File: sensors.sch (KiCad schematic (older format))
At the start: 23 parts, among them M1 ANEOMETER, U2 ADS1120-PW, U5 MPL115A1

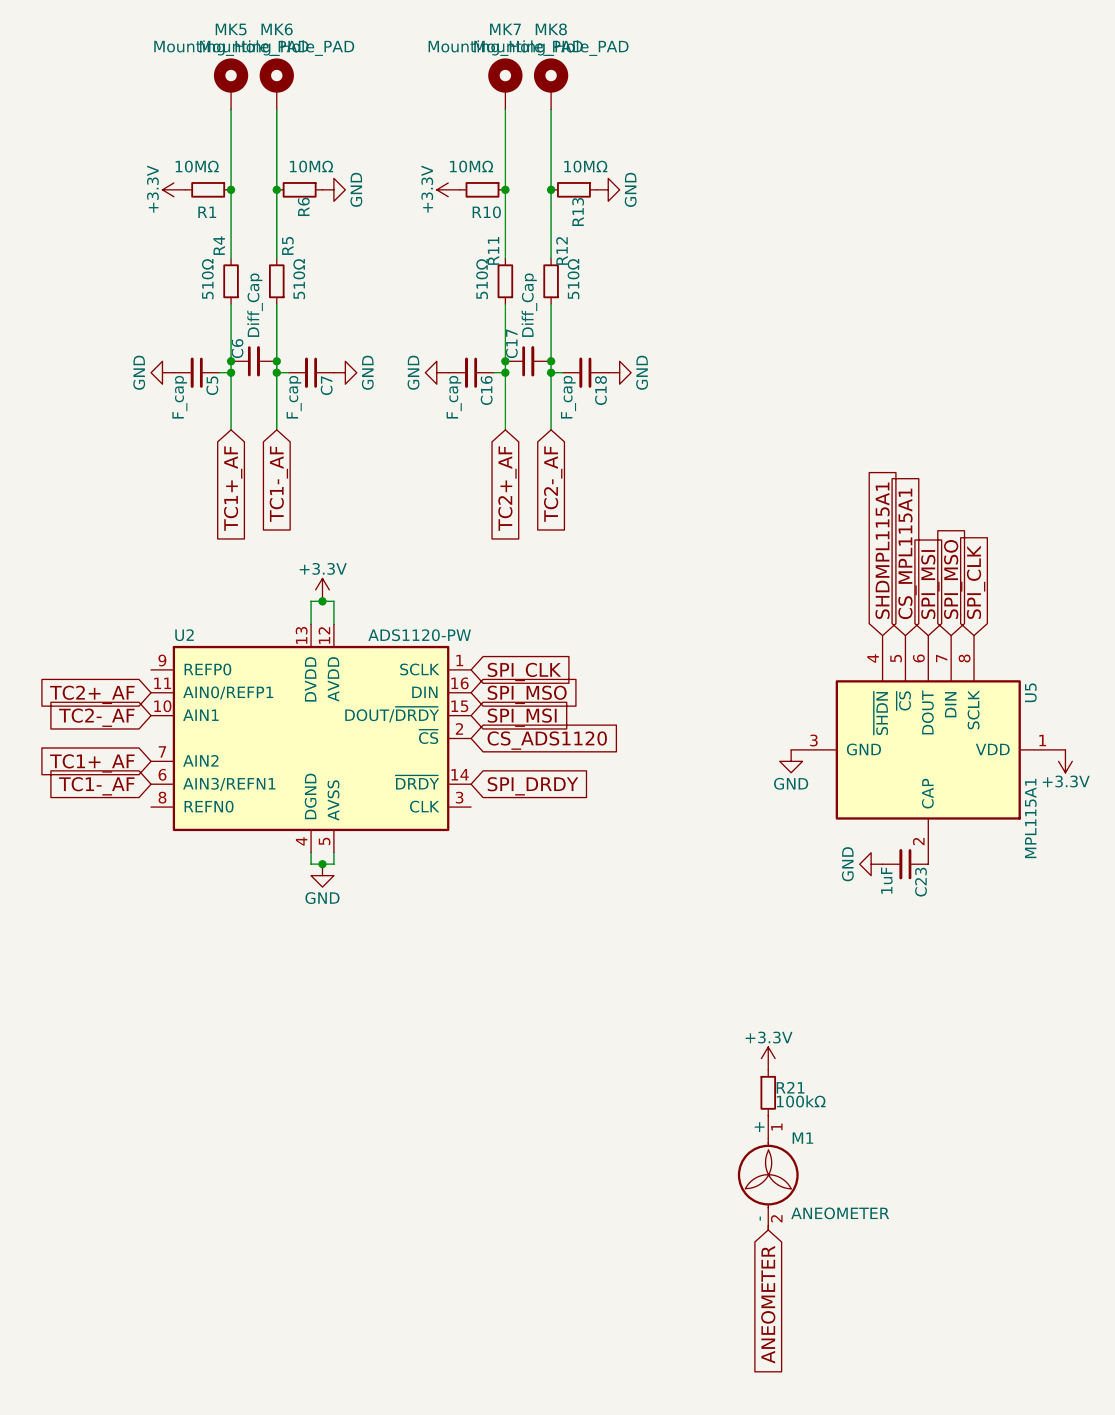
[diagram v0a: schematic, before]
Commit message: some changes
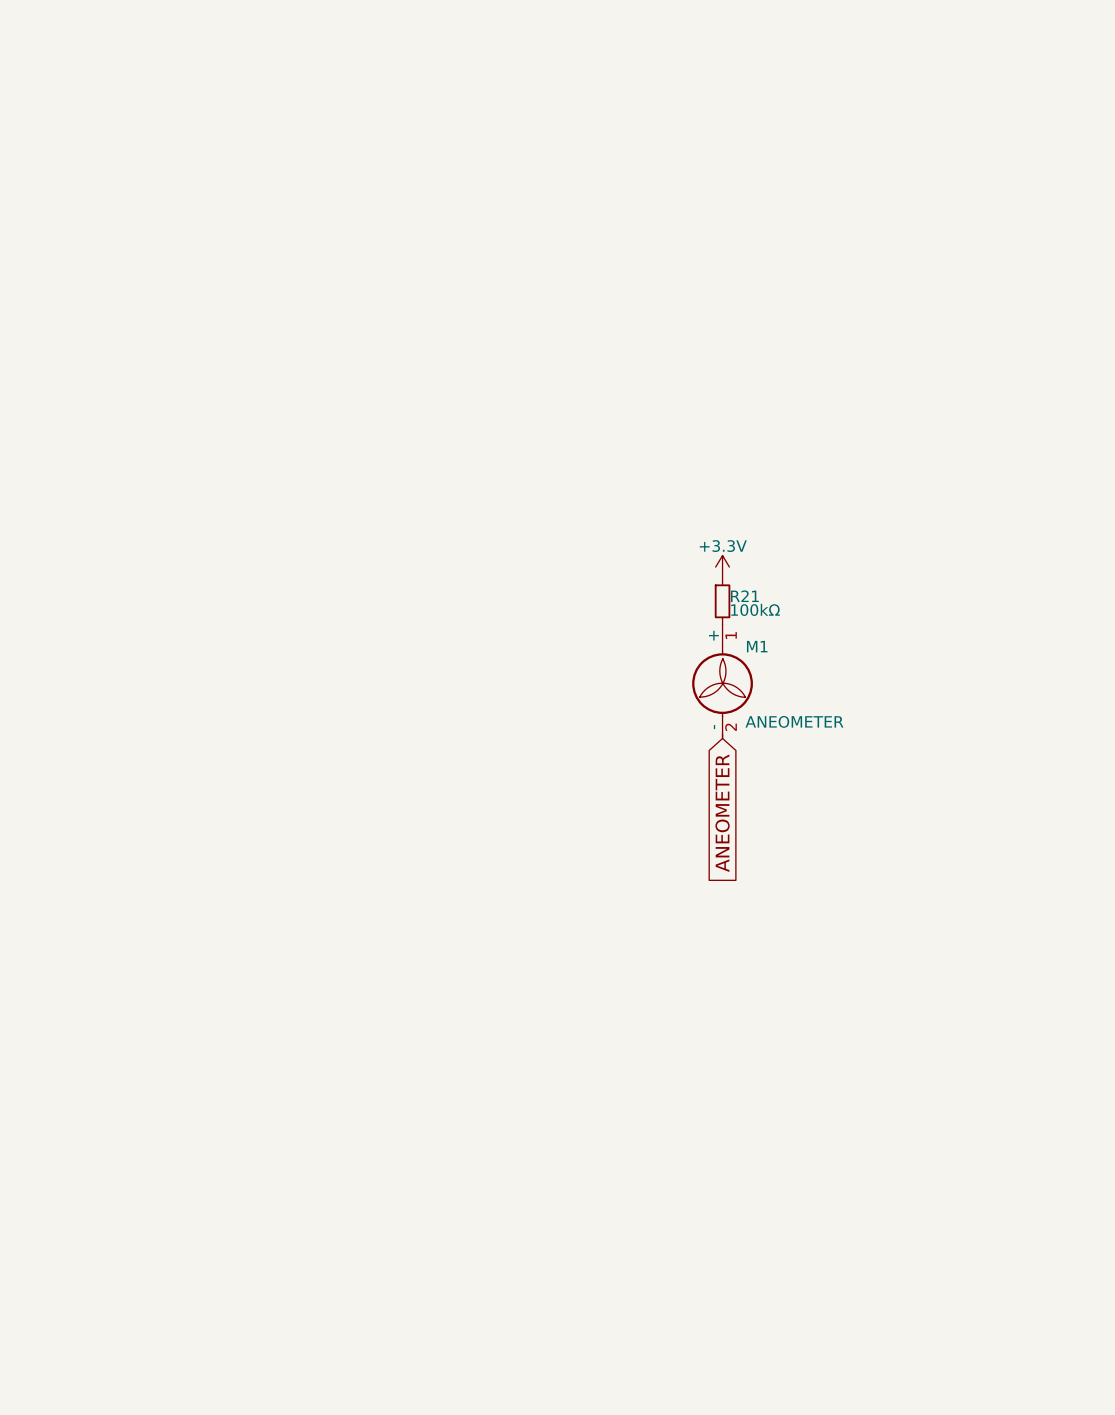
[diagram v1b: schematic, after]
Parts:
- removed C16, C18, C5, C7: F_cap, Capacitors_SMD:C_0402, symbol C_Small
- removed C17, C6: Diff_Cap, Capacitors_SMD:C_0402, symbol C_Small
- removed C23: 1uF, Capacitors_SMD:C_0402, symbol C_Small
- removed MK5, MK6, MK7, MK8: Mounting_Hole_PAD, Measurement_Points:Measurement_Point_Square-SMD-Pad_Big, symbol Mounting_Hole_PAD
- removed R1, R10, R13, R6: 10MΩ, Resistors_SMD:R_0603, symbol R_Small
- removed R11, R12, R4, R5: 510Ω, Resistors_SMD:R_0603, symbol R_Small
- removed U2: ADS1120-PW, Housings_SSOP:TSSOP-16_4.4x5mm_Pitch0.65mm, symbol ADS1120-PW
- removed U5: MPL115A1, Housings_LGA:LGA-8_3x5mm_Pitch1.25mm, symbol MPL115A1
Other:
- moved on the sheet: M1, R21
